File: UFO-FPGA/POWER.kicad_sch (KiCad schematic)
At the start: 33 parts, among them J5 USB_B_Micro, Q1 2N7002, U6 PWR convert, U7 PWR convert

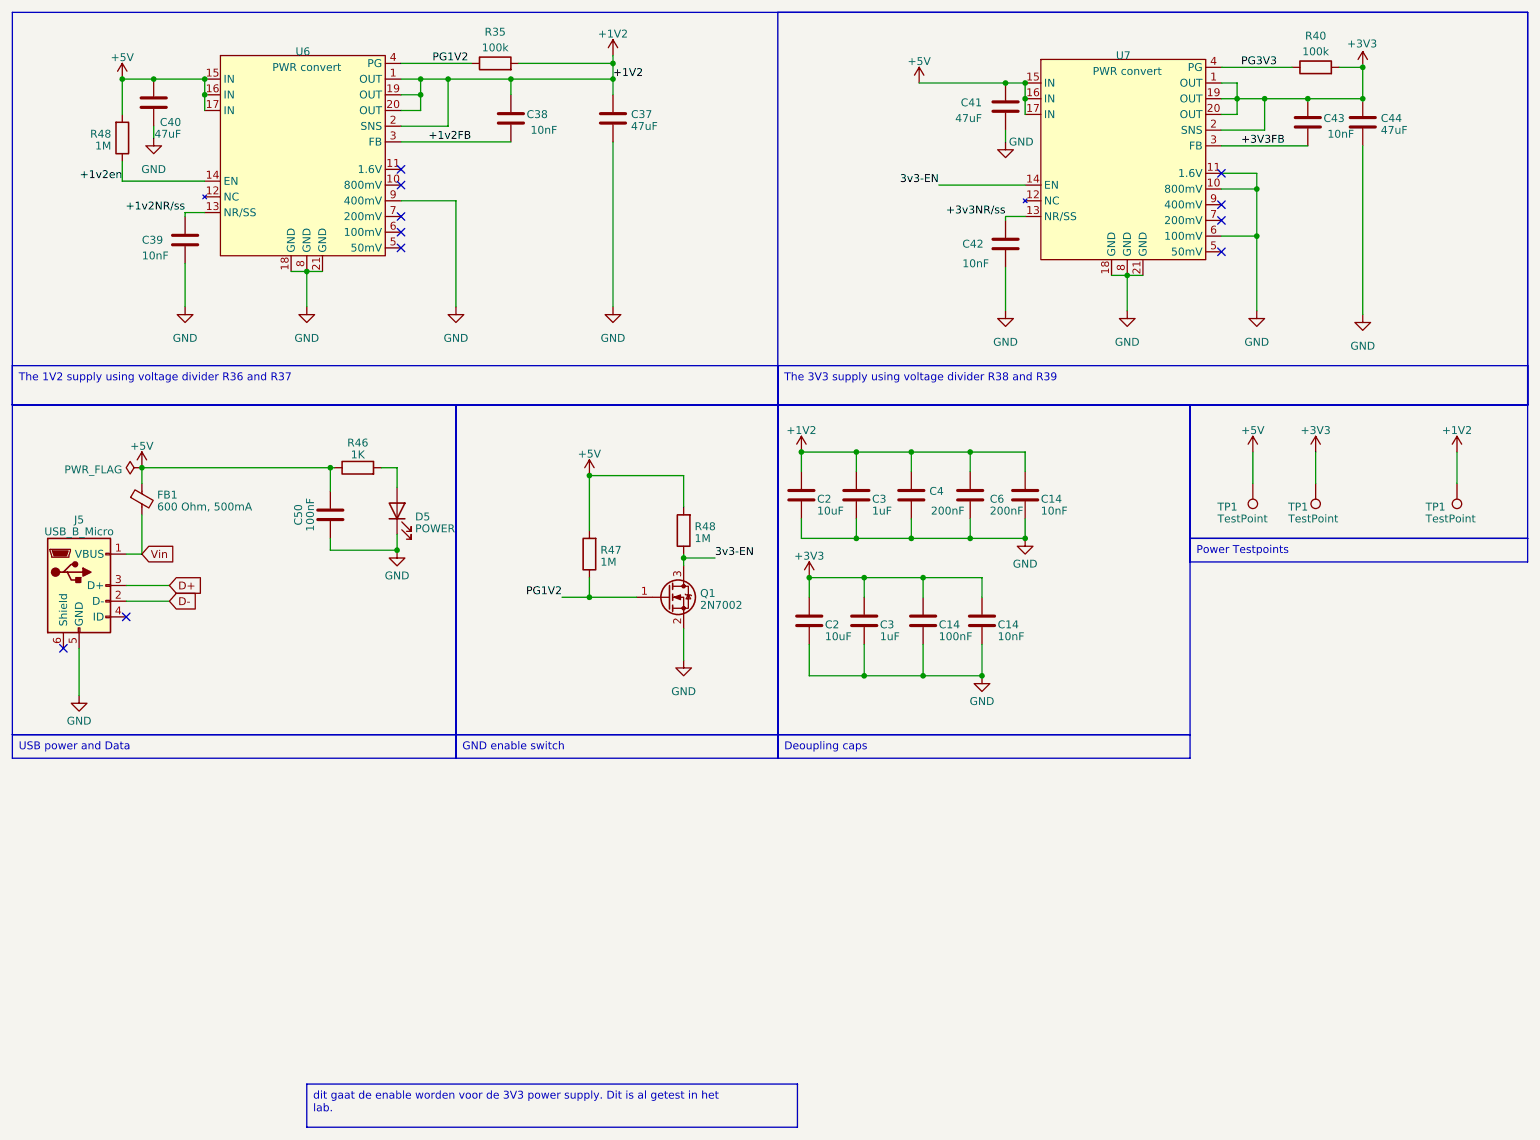
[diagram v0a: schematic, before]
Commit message: pcb
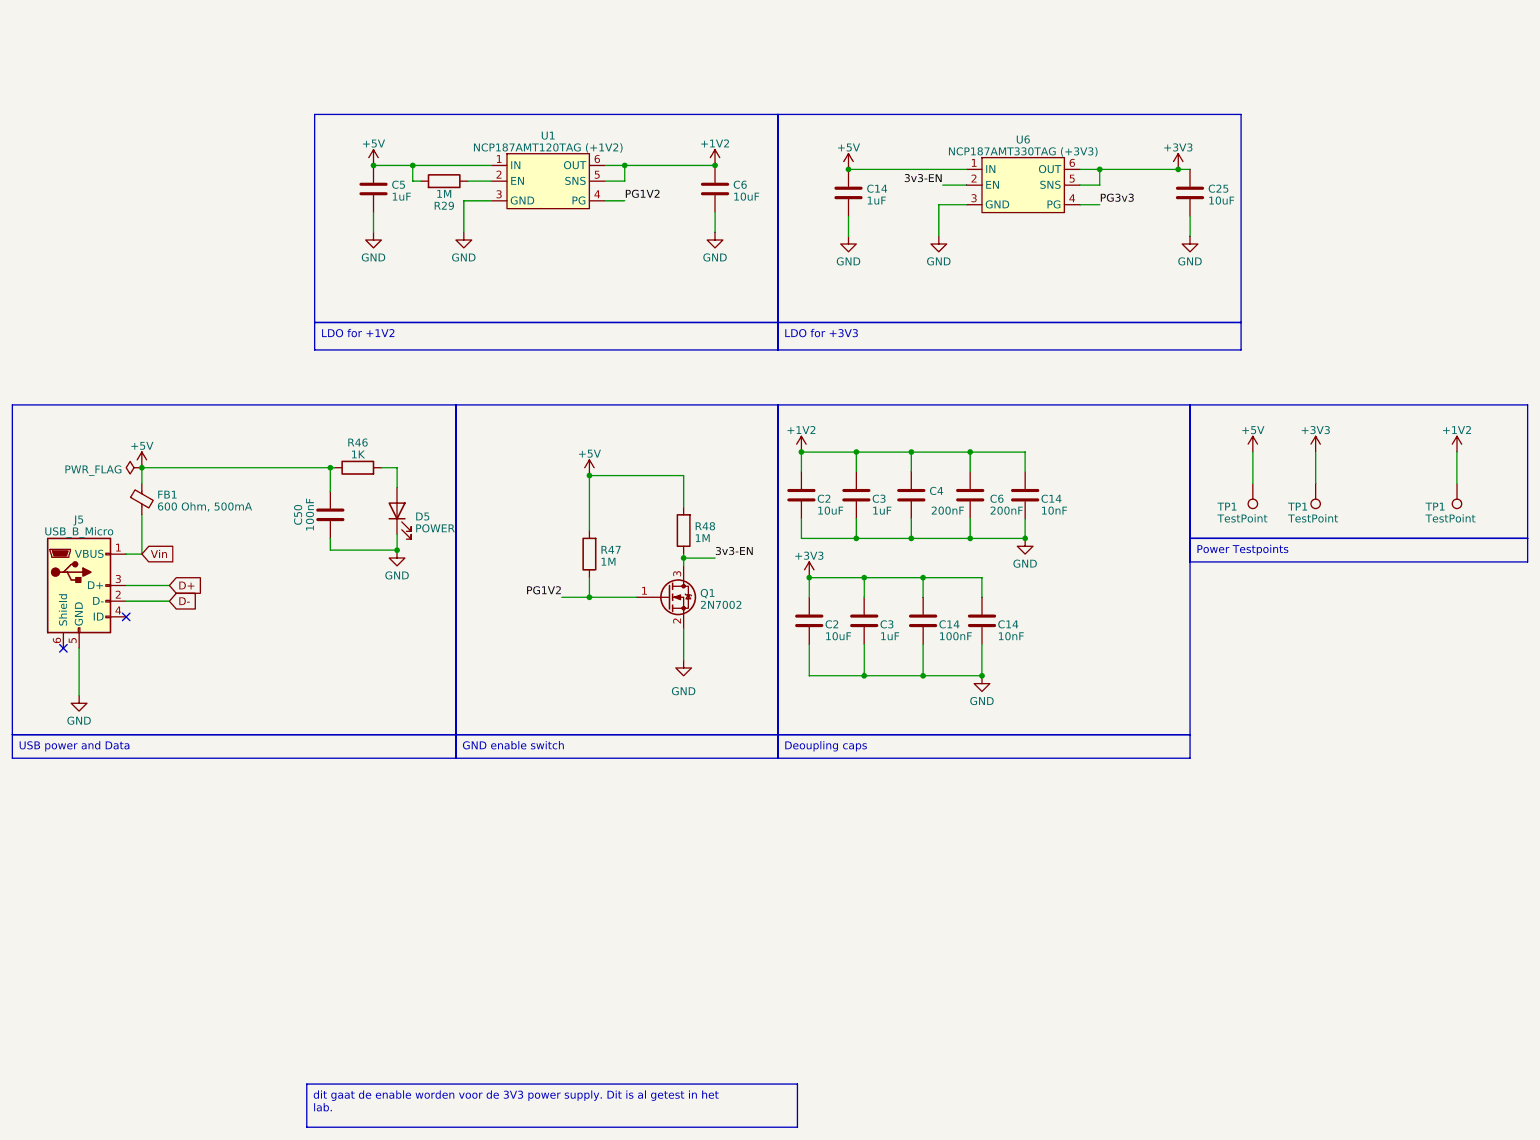
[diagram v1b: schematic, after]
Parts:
- removed C37, C40, C41, C44: 47uF, Capacitor_SMD:C_1206_3216Metric_Pad1.33x1.80mm_HandSolder, symbol Device:C
- removed C38, C39, C42, C43: 10nF, Capacitor_SMD:C_0603_1608Metric_Pad1.08x0.95mm_HandSolder, symbol Device:C
- removed R35: 100k, Resistor_SMD:R_0805_2012Metric_Pad1.20x1.40mm_HandSolder, symbol Device:R
- removed R40: 100k, Resistor_SMD:R_0805_2012Metric, symbol Device:R
- removed R48: 1M, Resistor_SMD:R_0805_2012Metric_Pad1.20x1.40mm_HandSolder, symbol Device:R
- removed U6, U7: PWR convert, UFO-Footpints:W-QFN3535-20, symbol UFO_PARTS:AP7179D-13
- added C14, C5: 1uF, Capacitor_SMD:C_0805_2012Metric_Pad1.18x1.45mm_HandSolder, symbol Device:C
- added C25, C6: 10uF, Capacitor_SMD:C_0805_2012Metric_Pad1.18x1.45mm_HandSolder, symbol Device:C
- added R29: 1M, Resistor_SMD:R_0805_2012Metric_Pad1.20x1.40mm_HandSolder, symbol Device:R
- added U1: NCP187AMT120TAG (+1V2), Package_DFN_QFN:DFN-6-1EP_2x2mm_P0.65mm_EP1x1.6mm, symbol UFO_PARTS:NCP187AMT120TAG (+1V2)
- added U6: NCP187AMT330TAG (+3V3), Package_DFN_QFN:DFN-6-1EP_2x2mm_P0.65mm_EP1x1.6mm, symbol UFO_PARTS:NCP187AMT330TAG (+3V3)
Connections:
- net +1V2: now also C6.1, U1.5 (SNS), U1.6 (OUT)
- net +3V3: now also C25.1, U6.5 (SNS), U6.6 (OUT)
- net +5V: now also C14.1, C5.1, R29.2, U1.1 (IN), U6.1 (IN)
- net 3v3-EN: now also U6.2 (EN)
- net GND: now also C14.2, C25.2, C5.2, C6.2, U1.3 (GND), U6.3 (GND)
- net PG1V2: now also U1.4 (PG)
- new net: R29.1, U1.2 (EN)
- new net PG3v3: U6.4 (PG)
- no-connect marks 11 -> 2
